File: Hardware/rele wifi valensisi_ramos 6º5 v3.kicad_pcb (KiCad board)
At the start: 2 copper layers, 125.1 x 140.5 mm, 45 parts, among them J1 relay-1, J2 relay-2, J3 relay-3, J4 relay-4, J5 entrada, J6 relay-1.1, J7 relay-2.2, J8 relay-3.3, J9 relay-4.4, K1 Relay_DPDT, K2 Relay_DPDT, K3 Relay_DPDT, K4 Relay_DPDT, Q1 2N2222, Q2 2N2222, Q3 2N2222, Q4 2N2222, U1 PC817, U2 PC817, U3 PC817, U4 PC817, U6 L7805, U7 ESP32_DEVKITC

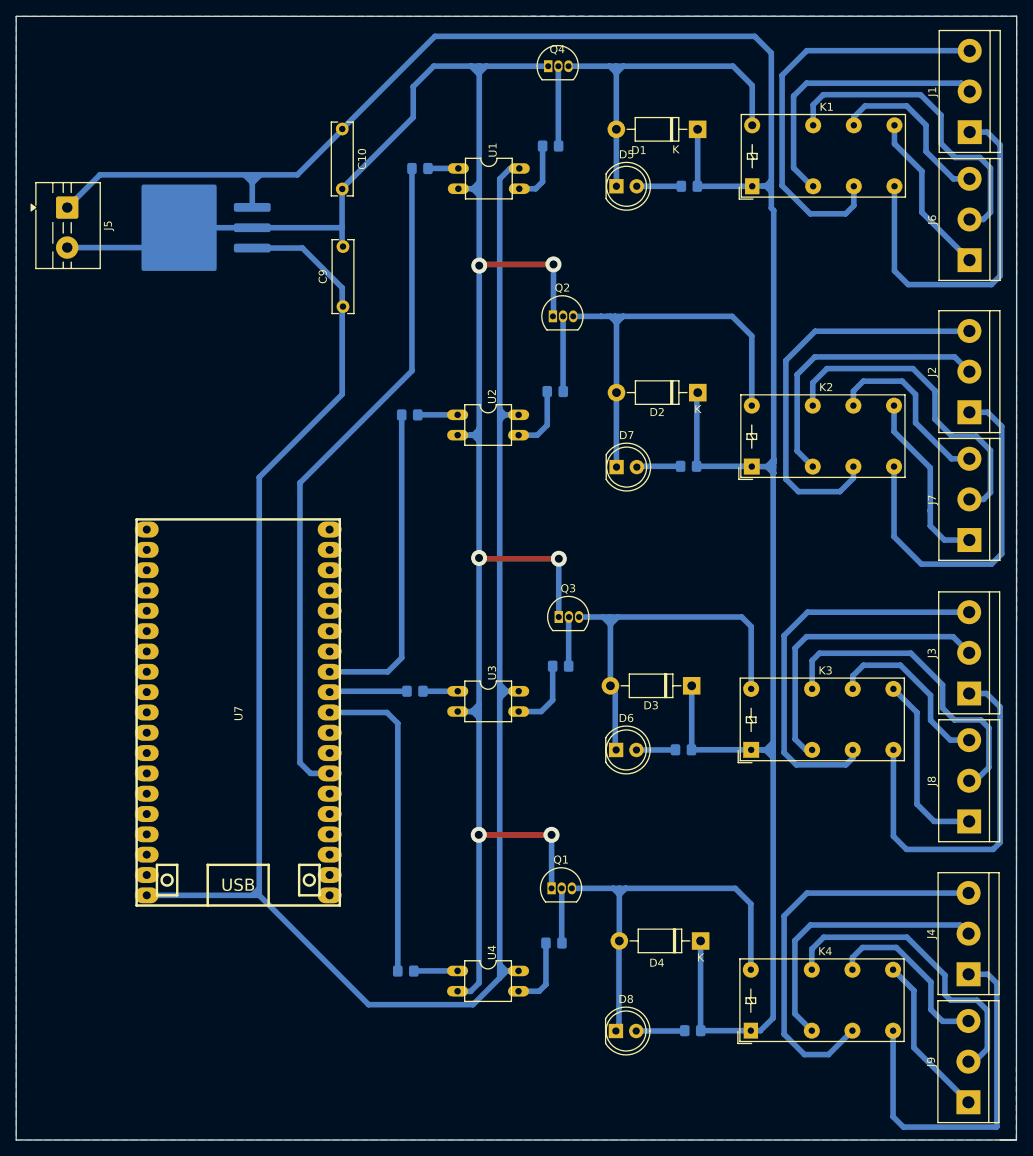
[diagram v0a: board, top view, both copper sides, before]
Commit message: Add files via upload
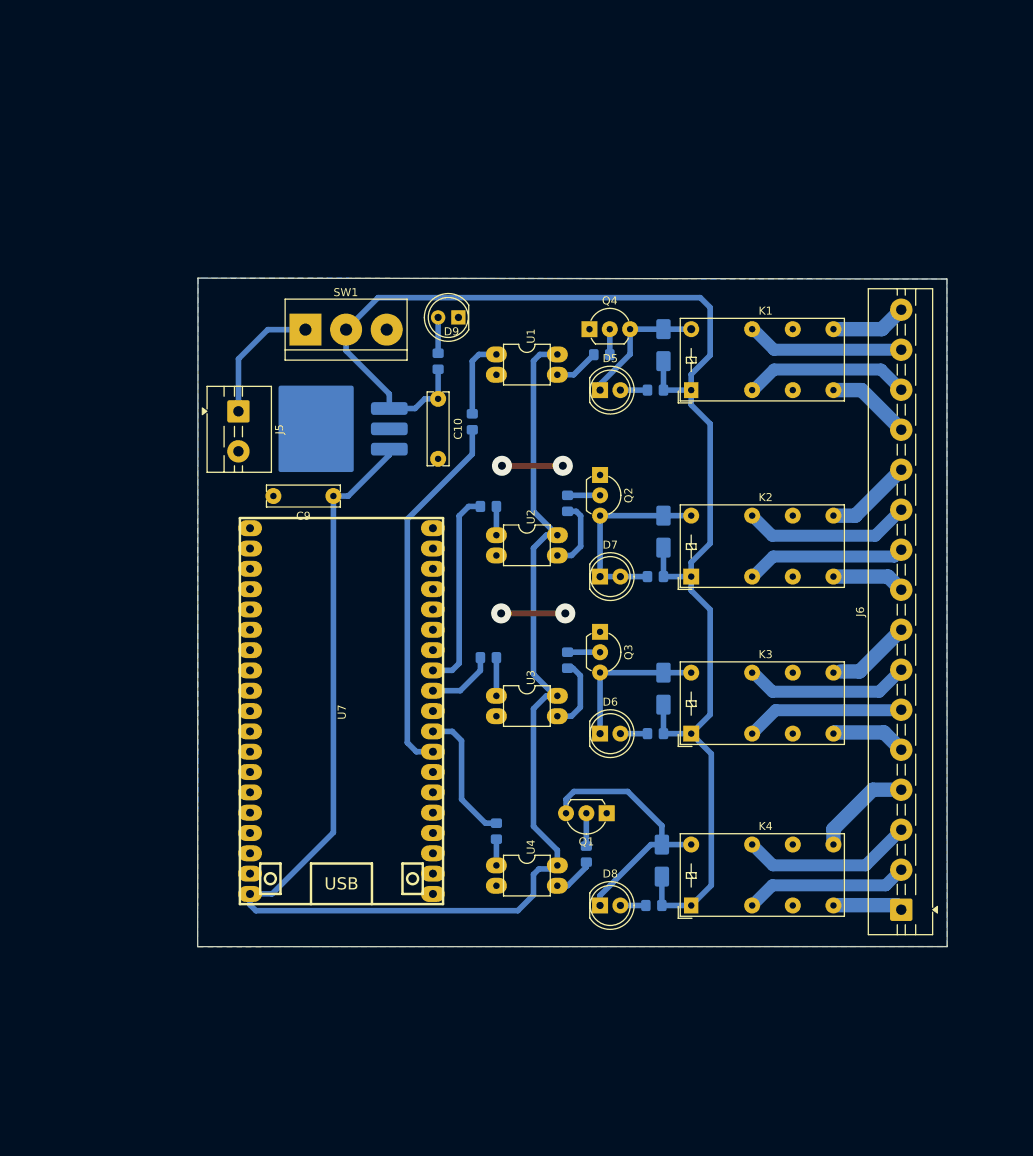
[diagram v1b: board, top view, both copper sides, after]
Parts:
- removed J1: relay-1, TerminalBlock:TerminalBlock_bornier-3_P5.08mm
- removed J2: relay-2, TerminalBlock:TerminalBlock_bornier-3_P5.08mm
- removed J3: relay-3, TerminalBlock:TerminalBlock_bornier-3_P5.08mm
- removed J4: relay-4, TerminalBlock:TerminalBlock_bornier-3_P5.08mm
- removed J7: relay-2.2, TerminalBlock:TerminalBlock_bornier-3_P5.08mm
- removed J8: relay-3.3, TerminalBlock:TerminalBlock_bornier-3_P5.08mm
- removed J9: relay-4.4, TerminalBlock:TerminalBlock_bornier-3_P5.08mm
- added D9: LED, LED_THT:LED_D5.0mm, F.Cu at (125.3, 56.4)
- added R13: 470, Resistor_SMD:R_0805_2012Metric_Pad1.20x1.40mm_HandSolder, B.Cu at (122.8, 61.8)
- added SW1: SW_DPST_x2, TerminalBlock:TerminalBlock_bornier-3_P5.08mm, F.Cu at (106.2, 57.9)
- D1, D2, D3, D4: footprint Diode_THT:D_DO-41_SOD81_P10.16mm_Horizontal -> Diode_SMD:D_SMA; moved to B.Cu
- J6: value relay-1.1 -> Screw_Terminal_01x16; footprint TerminalBlock:TerminalBlock_bornier-3_P5.08mm -> TerminalBlock:TerminalBlock_MaiXu_MX126-5.0-16P_1x16_P5.00mm
- Q1, Q2, Q3: footprint Package_TO_SOT_THT:TO-92L_Inline -> Package_TO_SOT_THT:TO-92L_Inline_Wide
- Q4: footprint Package_TO_SOT_THT:TO-92L_Inline -> Package_TO_SOT_THT:TO-92_Inline_Wide
- moved J6 81.6 mm to (180.6, 130.4)
- moved C10 35.8 mm to (122.8, 66.5)
- moved Q4 33.3 mm to (141.7, 57.8)
- moved J5 33.3 mm to (97.8, 68.1)
- moved R2 32.3 mm to (127.0, 69.4), turned to 90 degrees
- moved U6 30.4 mm to (109.0, 70.3)
- moved D1 27.3 mm to (150.9, 59.8), turned to 90 degrees
- moved R1 26.9 mm to (143.2, 61.0)
- moved K1 26.6 mm to (154.4, 65.5)
- moved R9 25.8 mm to (149.9, 65.5)
- moved D5 25.6 mm to (143.0, 65.5)
- moved U1 23.7 mm to (133.8, 62.3)
- moved C9 23.7 mm to (109.7, 78.7), turned to 180 degrees
- moved R7 20.8 mm to (130.0, 120.6), turned to -90 degrees
- moved Q2 20.7 mm to (143.0, 76.1), turned to -90 degrees
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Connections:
- J5 pad 1: +12V -> Net-(J1-Pin_2)
- J6 pad 1: NO-1.1 -> NO-4
- J6 pad 2: COM-1.1 -> COM-4
- J6 pad 3: NC-1.1 -> COM-4.4
- R2 pad 1: P4 -> P16
- R7 pad 1: P5 -> P17
- U7 pad 26: P4 -> unconnected-(U7-IO4-Pad26)
- U7 pad 27: unconnected-(U7-IO16-Pad27) -> P16
- U7 pad 28: unconnected-(U7-IO17-Pad28) -> P17
- U7 pad 29: P5 -> unconnected-(U7-IO5-Pad29)
- U7 pad 38: unconnected-(U7-GND-Pad38) -> GND
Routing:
- net GND: track 263.0 -> 15.6 mm, vias 6 -> 4
- net +12V: track 307.4 -> 179.2 mm
- net P4: track 84.3 -> 0.00 mm
- net +5V: track 262.7 -> 184.1 mm
- net NC-1: track 51.8 -> 0.00 mm
- net NC-2: track 50.5 -> 0.00 mm
- net NC-4: track 49.9 -> 0.00 mm
- net NC-3: track 49.6 -> 0.00 mm
- net P16: track 0.00 -> 46.1 mm
- net P5: track 40.1 -> 0.00 mm
- net NO-4: track 46.2 -> 8.73 mm
- net NO-3: track 46.7 -> 9.44 mm
- net NO-2: track 44.9 -> 9.04 mm
- net NO-1: track 45.8 -> 10.4 mm
- net Net-(D2-A): track 53.3 -> 19.1 mm
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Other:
- board size 125.1 x 140.5 mm -> 93.7 x 83.6 mm
